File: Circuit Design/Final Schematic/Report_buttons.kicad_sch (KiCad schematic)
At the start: 6 parts

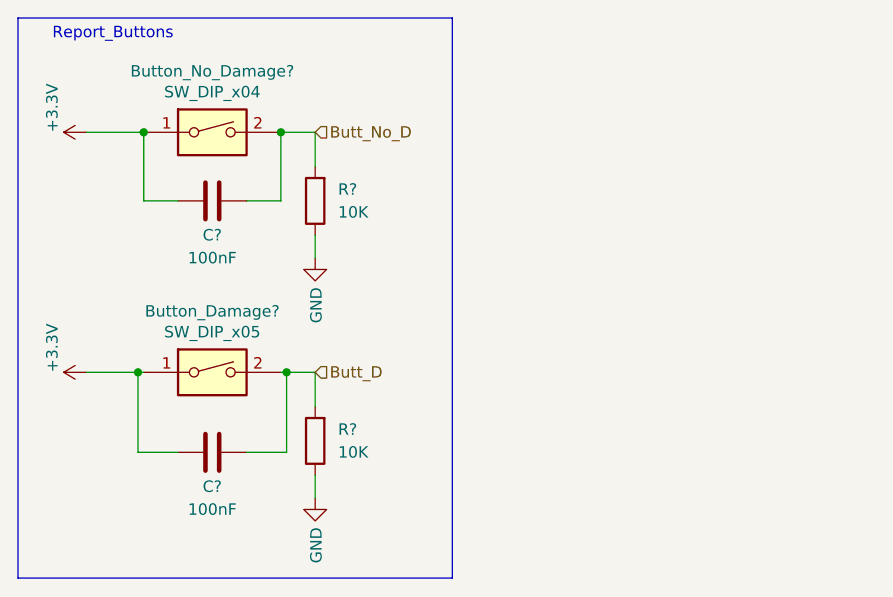
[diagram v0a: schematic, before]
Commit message: Footprints
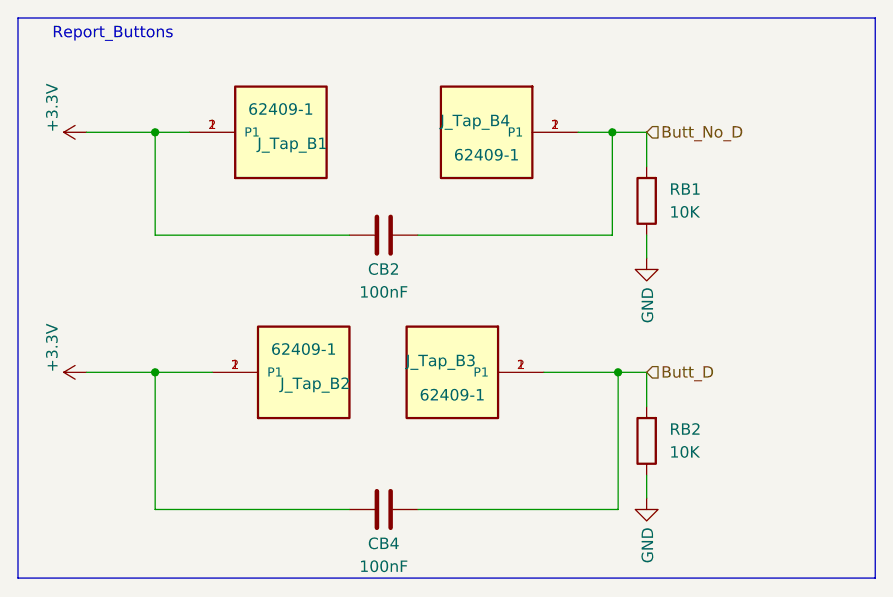
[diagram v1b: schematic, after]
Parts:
- removed Button_Damage?: SW_DIP_x05, symbol Switch:SW_DIP_x01
- removed Button_No_Damage?: SW_DIP_x04, symbol Switch:SW_DIP_x01
- added J_Tap_B1, J_Tap_B2, J_Tap_B3, J_Tap_B4: 62409-1, TE_62409-1, symbol Connector_Faston:62409-1
- gave numbers to parts that had none: 4
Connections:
- net +3V3: now also J_Tap_B1.1 (P1), J_Tap_B1.2 (P1), J_Tap_B2.1 (P1), J_Tap_B2.2 (P1)
- net Butt_D: now also J_Tap_B3.1 (P1), J_Tap_B3.2 (P1)
- net Butt_No_D: now also J_Tap_B4.1 (P1), J_Tap_B4.2 (P1)
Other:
- moved on the sheet: CB2, CB4, RB1, RB2
